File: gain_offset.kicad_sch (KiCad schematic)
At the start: 42 parts, among them U3 AD8337BCPZ-REEL-ND, U4 LMH6551MA, U5 AD8337BCPZ-REEL-ND, U7 LMH6551MA

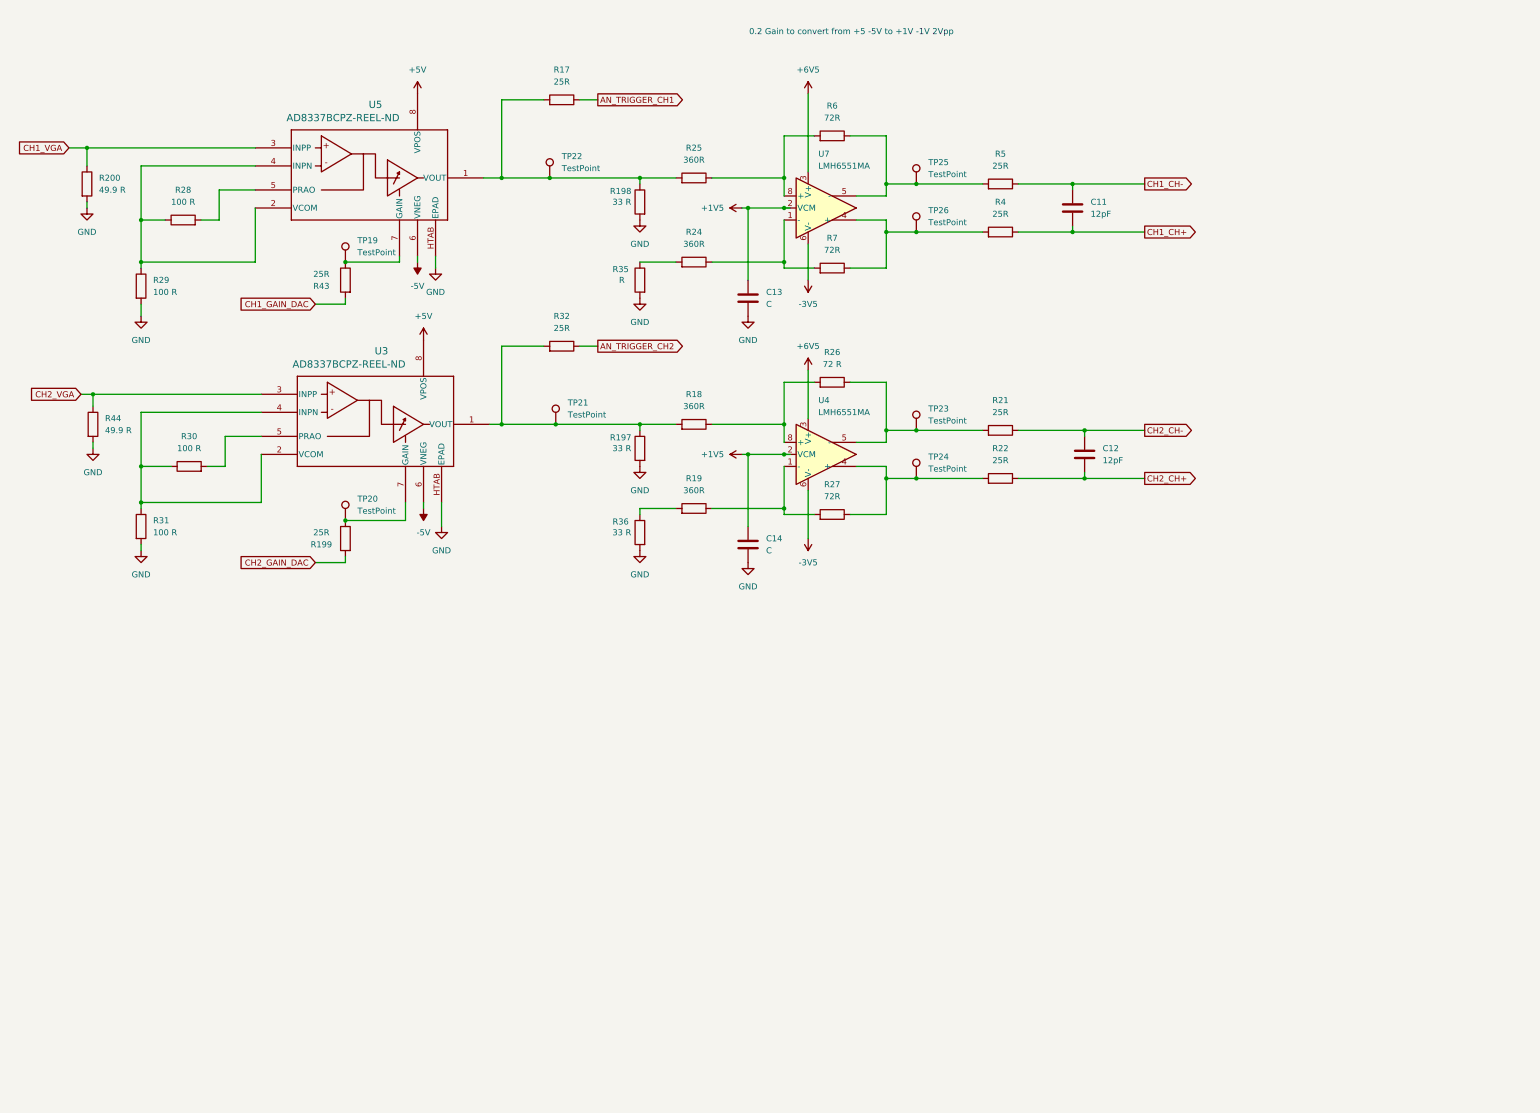
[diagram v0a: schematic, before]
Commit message: Finished schematic?
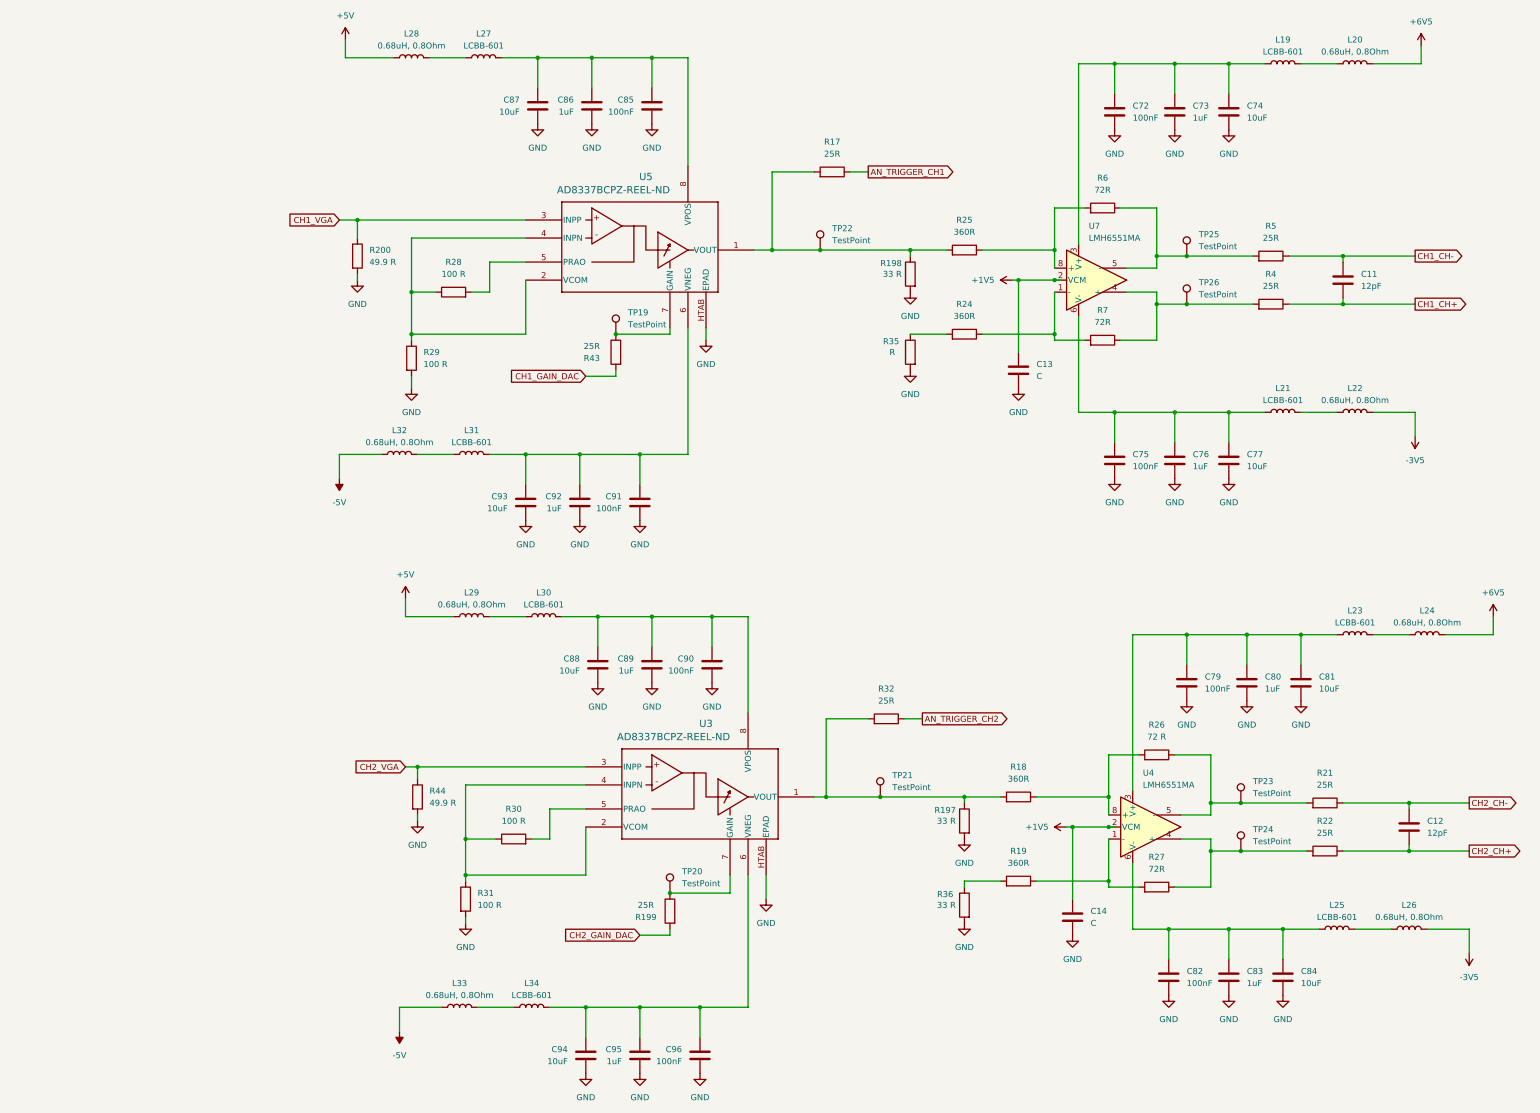
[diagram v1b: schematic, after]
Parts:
- added C72, C75, C79, C82, C85, C90, C91, C96: 100nF, symbol Device:C
- added C73, C76, C80, C83, C86, C89, C92, C95: 1uF, symbol Device:C
- added C74, C77, C81, C84, C87, C88, C93, C94: 10uF, symbol Device:C
- added L19, L21, L23, L25, L27, L30, L31, L34: LCBB-601, symbol Device:L
- added L20, L22, L24, L26, L28, L29, L32, L33: 0.68uH, 0.8Ohm, symbol Device:L
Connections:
- net +5V: now also L28.1, L29.1; no longer U3.8 (VPOS), U5.8 (VPOS)
- net +6V5: now also L20.1, L24.1; no longer U4.3 (V+), U7.3 (V+)
- net -3V5: now also L22.1, L26.1; no longer U4.6 (V-), U7.6 (V-)
- net -5V: now also L32.1, L33.1; no longer U3.6 (VNEG), U5.6 (VNEG)
- net GND: now also C72.2, C73.1, C74.1, C75.2, C76.1, C77.1, C79.2, C80.1, C81.1, C82.2, C83.1, C84.1, C85.2, C86.1, C87.1, C88.1, C89.1, C90.2, C91.2, C92.1, C93.1, C94.1, C95.1, C96.2
- new net: C91.1, C92.2, C93.2, L31.2, U5.6 (VNEG)
- new net: C85.1, C86.2, C87.2, L27.2, U5.8 (VPOS)
- new net: C75.1, C76.2, C77.2, L21.2, U7.6 (V-)
- new net: C79.1, C80.2, C81.2, L23.2, U4.3 (V+)
- new net: L29.2, L30.1
- new net: C94.2, C95.2, C96.1, L34.2, U3.6 (VNEG)
- new net: C72.1, C73.2, C74.2, L19.2, U7.3 (V+)
- new net: L25.1, L26.2
- new net: L21.1, L22.2
- new net: C88.2, C89.2, C90.1, L30.2, U3.8 (VPOS)
- new net: C82.1, C83.2, C84.2, L25.2, U4.6 (V-)
- new net: L33.2, L34.1
- new net: L27.1, L28.2
- new net: L31.1, L32.2
- new net: L23.1, L24.2
- new net: L19.1, L20.2
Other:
- note removed: "0.2 Gain to convert from +5 -5V to +1V -1V 2Vpp"
- moved on the sheet: C11, C12, C13, C14, R17, R18, R19, R197, R198, R199, R200, R21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
